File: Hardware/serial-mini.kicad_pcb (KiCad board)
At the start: 4 copper layers, 93 x 38.1 mm, 70 parts, among them J1 PICKIT V3 Header, J2 USB Micro B, J3 Serial Port, Q1 IRLML2060, Q2 IRLML2060, Q3 IRLML2060, U1 SIT2001BI-S2-33S-100.000000D, U2 FT230XQ-R, U3 DSPIC33CK64MP102, U4 SN74AHC14RGYR, U5 MIC5504-3.3YM5-TR

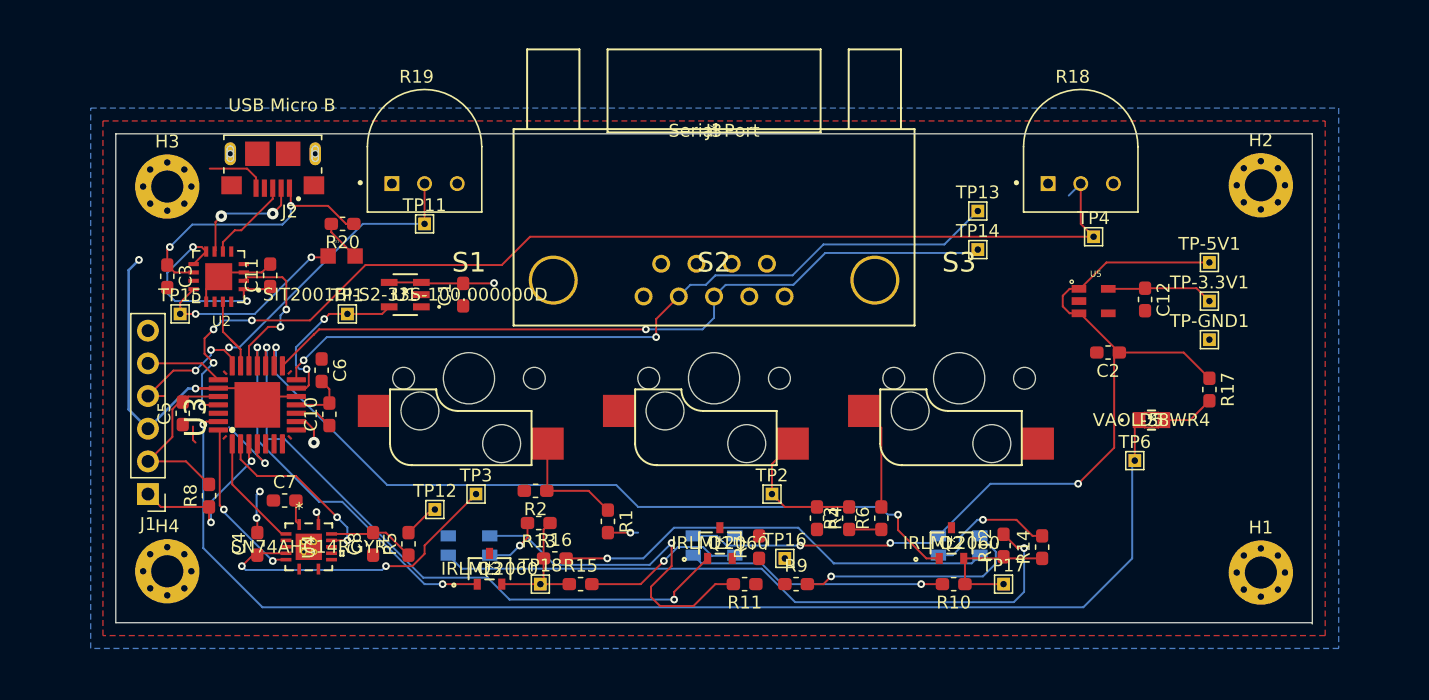
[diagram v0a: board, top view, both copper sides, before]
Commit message: Finish routing
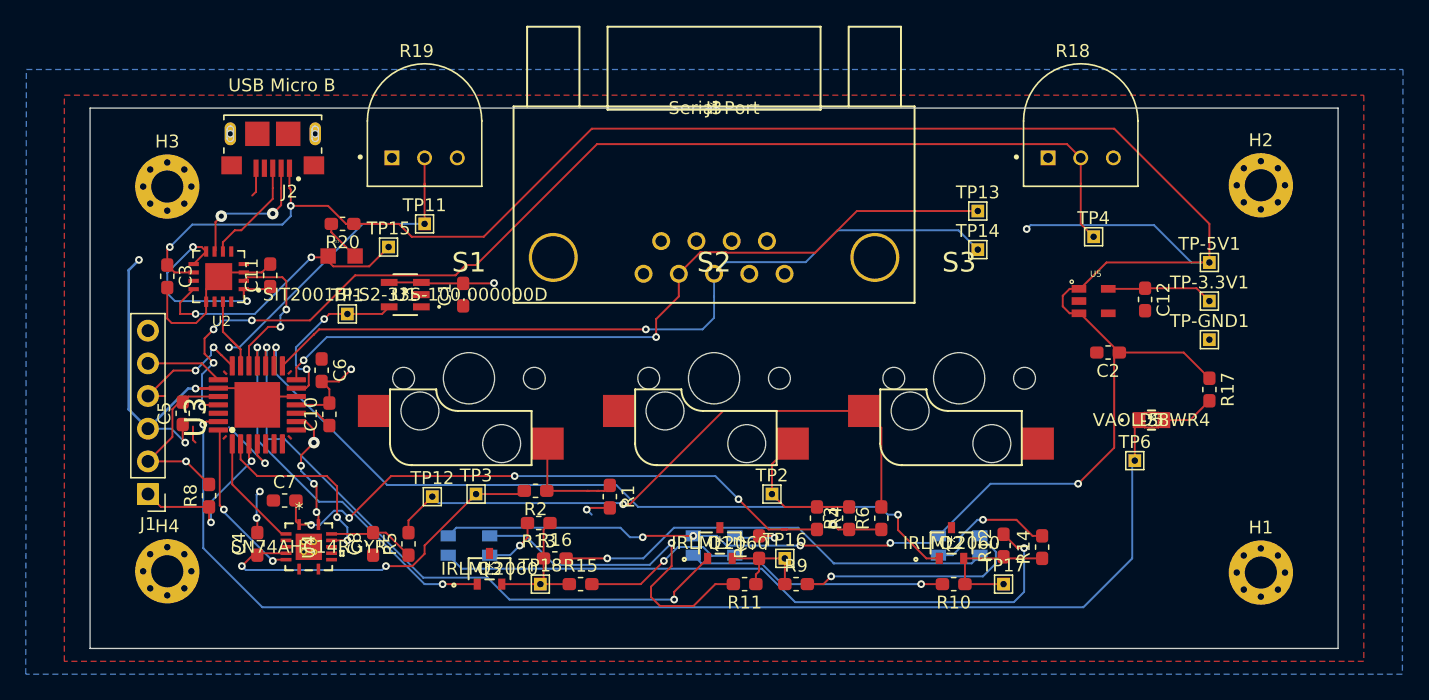
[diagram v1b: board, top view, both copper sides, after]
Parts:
- moved TP15 17.0 mm to (109.4, 80.0)
- moved R18 2.00 mm to (163.2, 70.2)
- moved R19 2.00 mm to (112.2, 70.2)
- moved R1 1.93 mm to (126.6, 99.4)
- moved J3 1.76 mm to (134.7, 69.2)
- moved J2 1.55 mm to (100.4, 71.2)
- moved TP12 1.02 mm to (112.8, 99.4)
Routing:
- net +5V: track 92.6 -> 205.8 mm, vias 5 -> 8
- net Net-(C7-Pad2): track 1.97 -> 46.4 mm, vias 0 -> 4
- net Net-(R5-Pad2): track 10.8 -> 48.4 mm, vias 0 -> 1
- net +3V3: track 43.9 -> 54.3 mm, vias 4 -> 9
- net GND: track 48.6 -> 57.7 mm, vias 4 -> 5
- net /1.7V@69mA: track 0.00 -> 8.20 mm
- net /3V@20mA: track 15.7 -> 21.6 mm
- net Net-(D2-Pad3): track 0.00 -> 4.41 mm, vias 0 -> 1
- net Net-(C4-Pad1): track 25.0 -> 28.8 mm
- net /PWM-Hue: track 85.5 -> 88.6 mm
- net TX: track 58.8 -> 61.4 mm
- net /PWM-Brightness: track 28.0 -> 30.1 mm
- net Net-(J2-Pad3): track 6.82 -> 8.37 mm
- net Net-(J2-Pad2): track 9.29 -> 10.8 mm
- net SWITCH_OUT_2: track 13.9 -> 15.3 mm
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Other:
- board size 93 x 38.1 mm -> 97 x 42 mm
